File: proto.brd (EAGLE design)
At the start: 160 x 100 mm, 7 parts

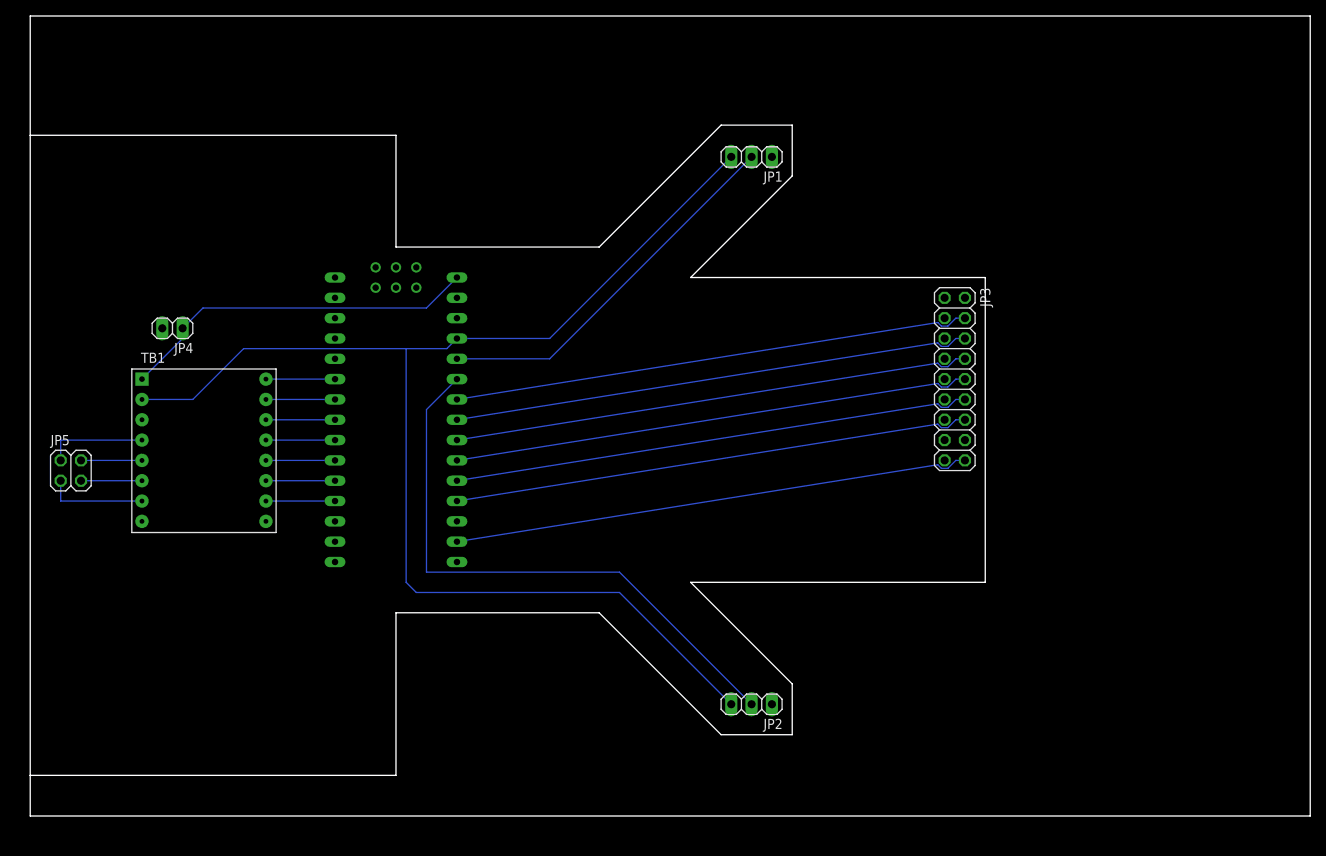
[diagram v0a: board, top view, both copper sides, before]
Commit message: monton de weas
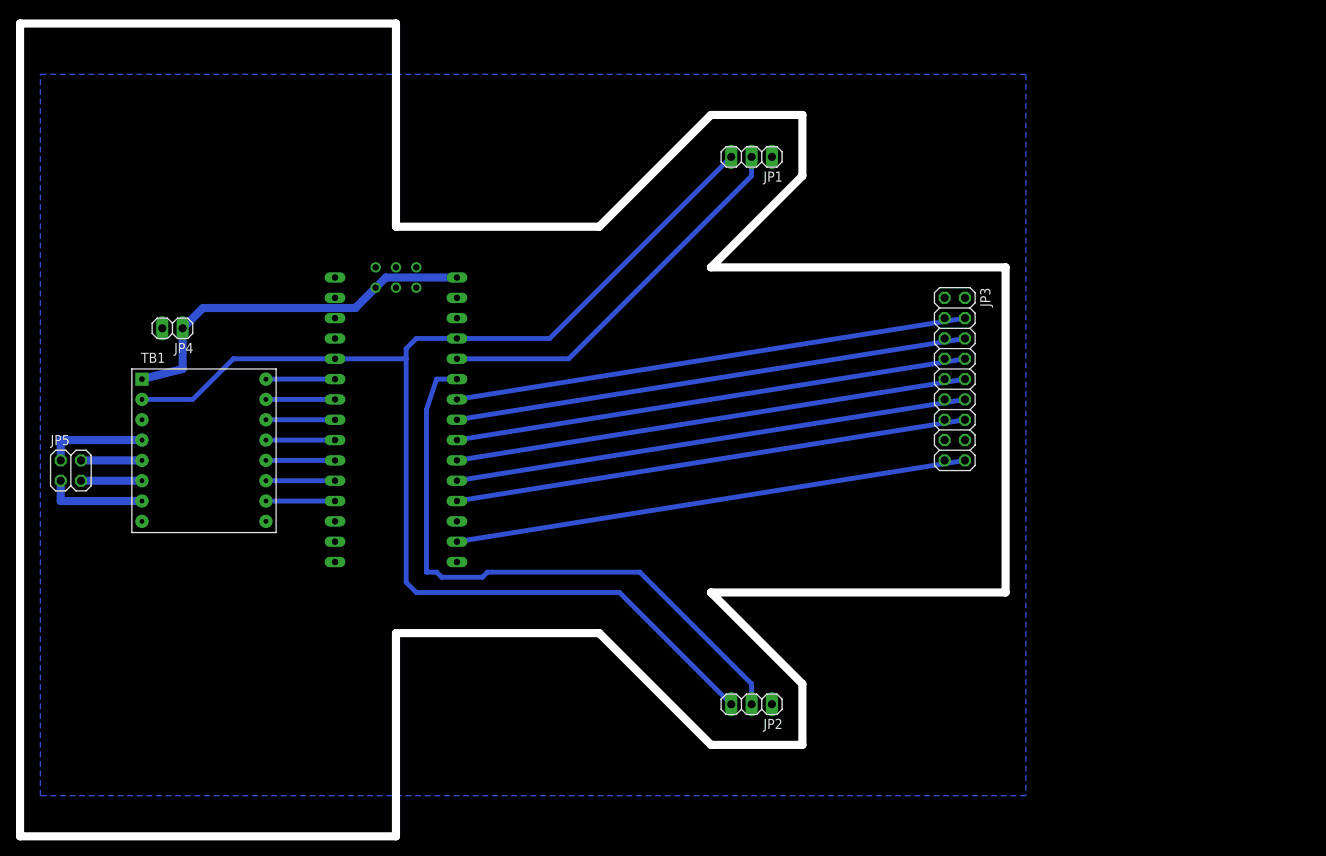
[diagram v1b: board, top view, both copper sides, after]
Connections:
- new net GND: JP1.1, JP2.1, JP3.1, JP4.2, TB1.GND2, TB1.GND3, U$1.GND, U$1.GND1
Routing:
- net N$26: track 73.2 -> 76.4 mm
- net N$9: track 45.4 -> 47.2 mm
- net N$17: track 47.3 -> 48.7 mm
- net N$18: track 64.9 -> 64.3 mm
- net N$16: track 64.9 -> 64.3 mm
- net N$15: track 64.9 -> 64.3 mm
- net N$14: track 64.9 -> 64.3 mm
- net N$20: track 64.9 -> 64.3 mm
- net N$19: track 64.9 -> 64.3 mm
- net N$10: track 64.9 -> 64.3 mm
- net N$27: track 162.4 -> 161.9 mm
- added copper zone on layer 16, net GND
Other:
- board size 160 x 100 mm -> 123.2 x 101.6 mm
